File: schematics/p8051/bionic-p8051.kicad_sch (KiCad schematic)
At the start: 10 parts, among them J1 Bionic-P135, J2 Bionic-P245, U1 P8051AH, U2 11AA010-I/TT

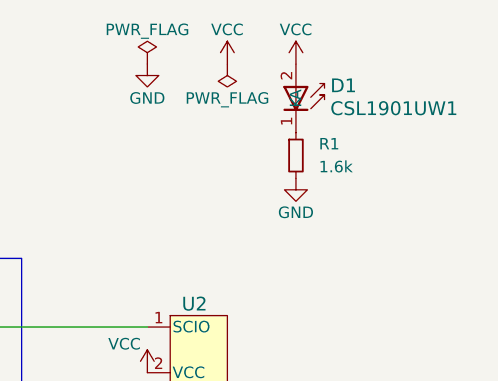
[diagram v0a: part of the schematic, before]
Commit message: [P8051] Cleanup schematics
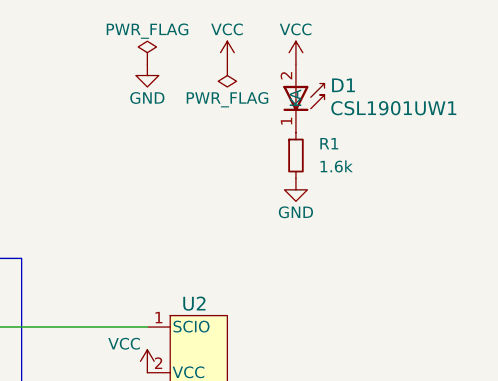
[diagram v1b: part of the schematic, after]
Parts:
- D1: footprint 0-LocalLibrary:LED_CSL1901UW1_ROM-M -> rhom:LED_CSL1901UW1_ROM-M; symbol 0-LocalLibrary:CSL1901UW1 -> rhom:CSL1901UW1
- J1: footprint 0-LocalLibrary:Bionic-P135_Vertical -> bionic:Bionic-P135_Vertical; symbol 0-LocalLibrary:Bionic-P135 -> bionic:Bionic-P135
- J2: footprint 0-LocalLibrary:Bionic-P245_Vertical -> bionic:Bionic-P245_Vertical; symbol 0-LocalLibrary:Bionic-P245 -> bionic:Bionic-P245
- JP1: footprint 0-LocalLibrary:SolderJumper-3_P1.3mm_Open_RoundedPad1.0x1.5mm_NumberLabels -> bionic:SolderJumper-3_P1.3mm_Open_RoundedPad1.0x1.5mm_NumberLabels
- JP2: footprint 0-LocalLibrary:SolderJumper-2_P1.3mm_Open_RoundedPad1.0x1.5mm -> bionic:SolderJumper-2_P1.3mm_Open_RoundedPad1.0x1.5mm
- U1: footprint 0-LocalLibrary:DIP-40_W15.24mm_Socket -> bionic:DIP-40_W15.24mm_Socket; symbol 0-LocalLibrary:P8051AH -> cpu:P8051AH
- U2: footprint 0-LocalLibrary:SOT-23_MC_MCH-M -> microchip:SOT-23_MC_MCH-M; symbol 0-LocalLibrary:11AA010-I_TT -> microchip:11AA010-I_TT
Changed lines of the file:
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@@
 			)
 		)
-		(property "Footprint" "0-LocalLibrary:SolderJumper-2_P1.3mm_Open_RoundedPad1.0x1.5mm"
+		(property "Footprint" "bionic:SolderJumper-2_P1.3mm_Open_RoundedPad1.0x1.5mm"
 			(at 64.77 104.14 0)
 			(effects
@@
 	)
 	(symbol
-		(lib_id "0-LocalLibrary:Bionic-P245")
+		(lib_id "bionic:Bionic-P245")
 		(at 179.07 99.06 0)
 		(unit 1)
@@
 			)
 		)
-		(property "Footprint" "0-LocalLibrary:Bionic-P245_Vertical"
+		(property "Footprint" "bionic:Bionic-P245_Vertical"
 			(at 180.34 134.62 0)
 			(effects
@@
 			)
 		)
-		(property "Description" ""
+		(property "Description" "Generic connector, single row, 01x24, script generated (kicad-library-utils/schlib/autogen/connector/)"
 			(at 179.07 99.06 0)
 			(effects
@@
 	)
 	(symbol
-		(lib_id "0-LocalLibrary:Bionic-P135")
+		(lib_id "bionic:Bionic-P135")
 		(at 171.45 99.06 0)
 		(unit 1)
@@
 			)
 		)
-		(property "Footprint" "0-LocalLibrary:Bionic-P135_Vertical"
+		(property "Footprint" "bionic:Bionic-P135_Vertical"
 			(at 172.72 134.62 0)
 			(effects
@@
 			)
 		)
-		(property "Description" ""
+		(property "Description" "Generic connector, single row, 01x24, script generated (kicad-library-utils/schlib/autogen/connector/)"
 			(at 171.45 99.06 0)
 			(effects
@@
 			)
 		)
-		(property "Footprint" "0-LocalLibrary:SolderJumper-3_P1.3mm_Open_RoundedPad1.0x1.5mm_NumberLabels"
+		(property "Footprint" "bionic:SolderJumper-3_P1.3mm_Open_RoundedPad1.0x1.5mm_NumberLabels"
 			(at 64.77 116.84 0)
 			(effects
@@
 	)
 	(symbol
-		(lib_id "0-LocalLibrary:CSL1901UW1")
+		(lib_id "rhom:CSL1901UW1")
 		(at 226.06 44.45 270)
 		(unit 1)
@@
 		(fields_autoplaced yes)
 		(property "Reference" "D1"
-			(at 229.87 46.863 90)
+			(at 229.87 46.8629 90)
 			(effects
 				(font
@@
 		)
 		(property "Value" "CSL1901UW1"
-			(at 229.87 49.403 90)
+			(at 229.87 49.4029 90)
 			(effects
 				(font
@@
 			)
 		)
-		(property "Footprint" "0-LocalLibrary:LED_CSL1901UW1_ROM-M"
+		(property "Footprint" "rhom:LED_CSL1901UW1_ROM-M"
 			(at 217.17 48.26 0)
 			(effects
@@
 	)
 	(symbol
-		(lib_id "0-LocalLibrary:11AA010-I_TT")
+		(lib_id "microchip:11AA010-I_TT")
 		(at 212.09 72.39 0)
 		(unit 1)
@@
 			)
 		)
-		(property "Footprint" "0-LocalLibrary:SOT-23_MC_MCH-M"
+		(property "Footprint" "microchip:SOT-23_MC_MCH-M"
 			(at 214.63 90.17 0)
 			(effects
@@
 			)
 		)
-		(property "Description" ""
+		(property "Description" "UNI/O Serial EEPROM (1Kbit)"
 			(at 212.09 72.39 0)
 			(effects
@@
 	)
 	(symbol
-		(lib_id "0-LocalLibrary:P8051AH")
+		(lib_id "cpu:P8051AH")
 		(at 110.49 101.6 0)
 		(unit 1)
@@
 			)
 		)
-		(property "Footprint" "0-LocalLibrary:DIP-40_W15.24mm_Socket"
+		(property "Footprint" "bionic:DIP-40_W15.24mm_Socket"
 			(at 111.76 135.89 0)
 			(effects
@@
 			)
 		)
-		(property "Description" ""
+		(property "Description" "8-bit General Purpose Microprocessor, DIP-40"
 			(at 110.49 101.6 0)
 			(effects
